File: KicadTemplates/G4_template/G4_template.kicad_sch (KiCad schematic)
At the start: 16 parts, among them J1 Conn_01x04_Female, SW1 SW_SPDT, U1 NUCLEO-G491RE

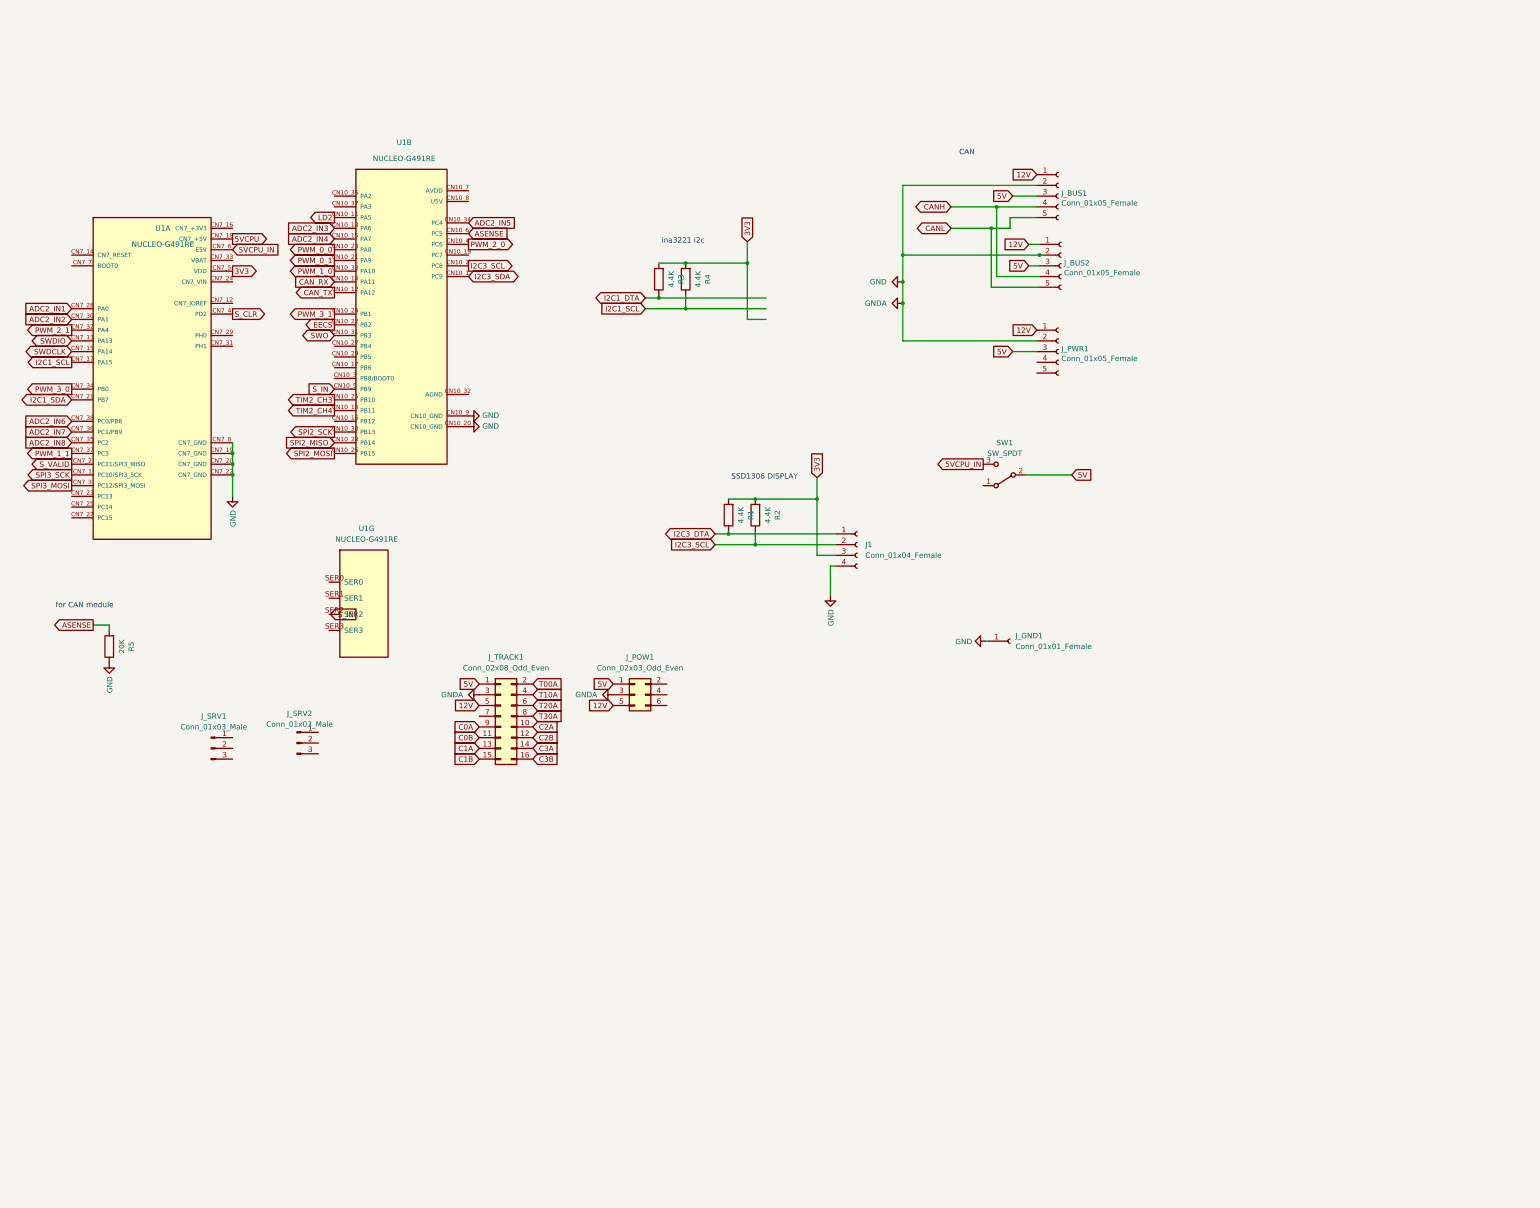
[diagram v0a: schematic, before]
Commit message: update spec POW_CTRL
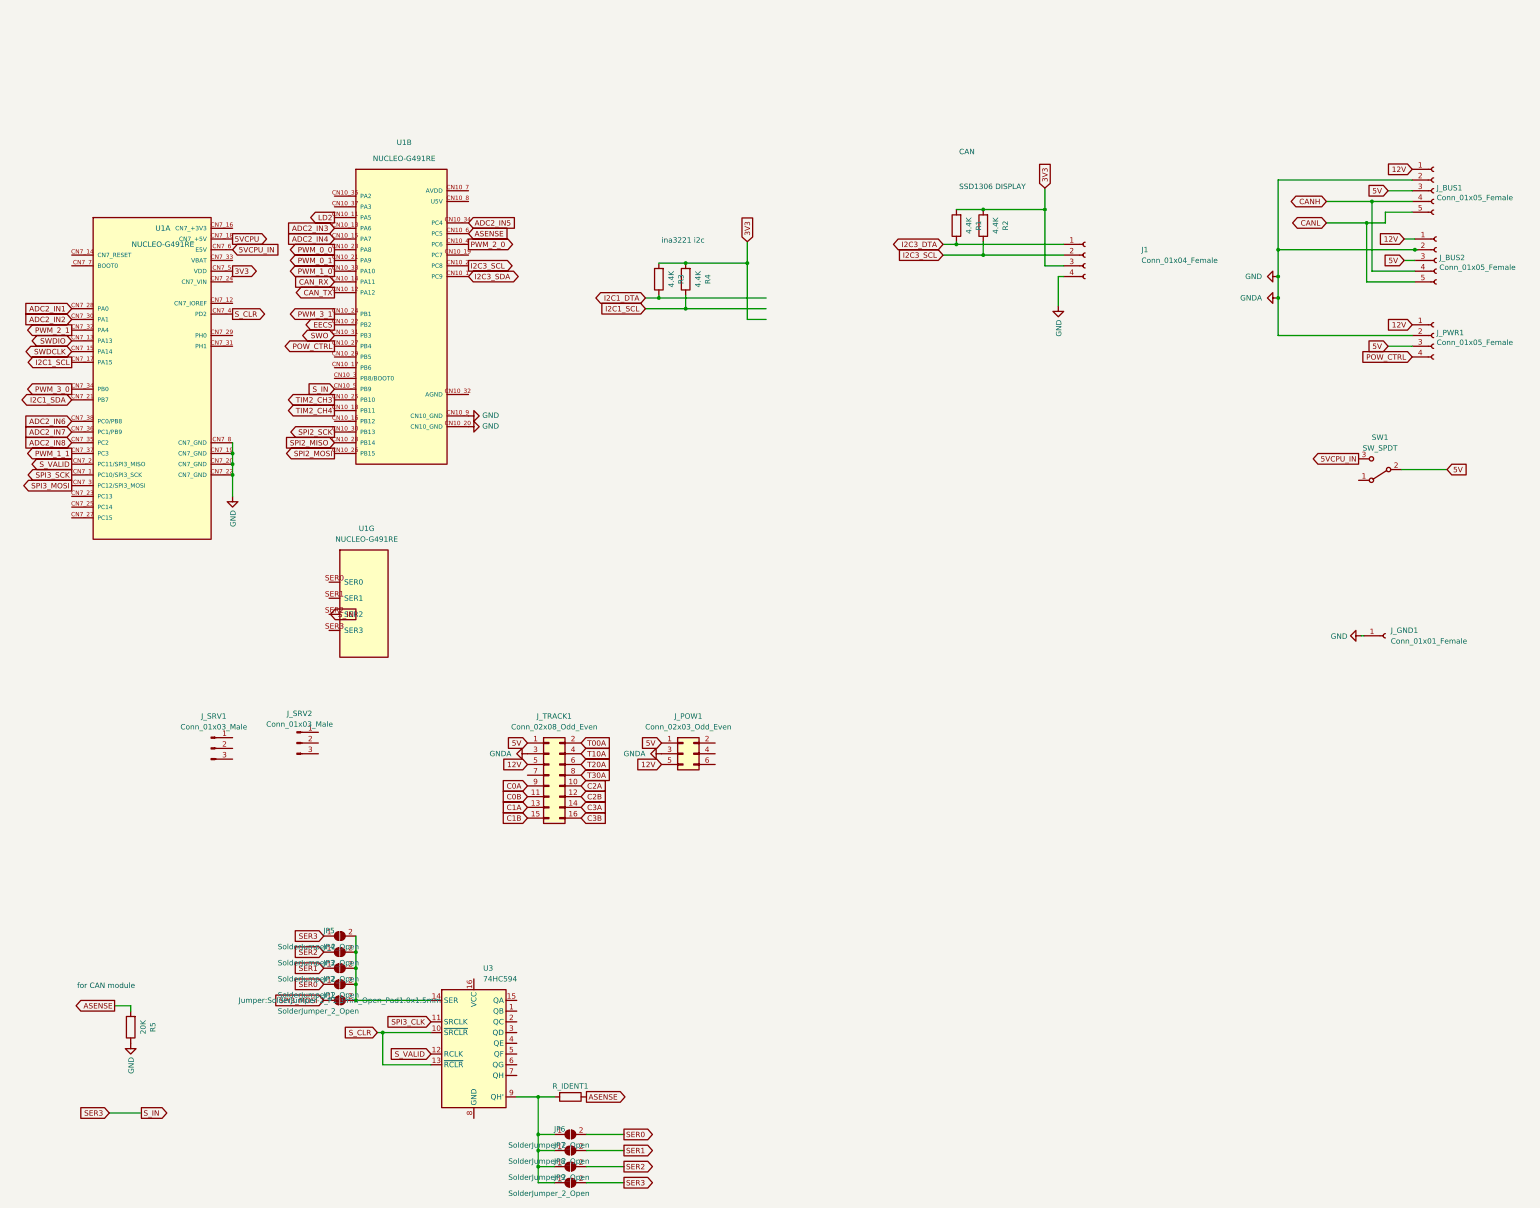
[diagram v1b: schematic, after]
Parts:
- added JP1, JP2, JP3, JP4, JP5, JP6, JP7, JP8, JP9: SolderJumper_2_Open, Jumper:SolderJumper-2_P1.3mm_Open_Pad1.0x1.5mm, symbol Jumper:SolderJumper_2_Open
- added R_IDENT1: ~, Resistor_THT:R_Axial_DIN0207_L6.3mm_D2.5mm_P7.62mm_Horizontal, symbol Device:R
- added U3: 74HC594, Package_DIP:DIP-16_W7.62mm_LongPads, symbol DBN:74HC594
- J_PWR1: footprint Connector_JST:JST_XH_S5B-XH-A_1x05_P2.50mm_Horizontal -> Connector_JST:JST_XH_S4B-XH-A-1_1x04_P2.50mm_Horizontal; symbol Connector:Conn_01x05_Female -> Connector:Conn_01x04_Socket
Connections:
- net ASENSE: now also R_IDENT1.1
- net SPI3_MOSI: now also JP1.1 (A)
- net S_CLR: now also U3.10 (~{SRCLR}), U3.13 (~{RCLR})
- net S_VALID: now also U3.12 (RCLK)
- net POW_CTRL: now reaches J_PWR1.4 (Pin_4)
- net POW_CTRL: now also U1.CN10_27 (PB4)
- net S_IN renamed SER3
- net SER3: now also JP5.1 (A), JP9.2 (B)
- new net: JP6.1 (A), JP7.1 (A), JP8.1 (A), JP9.1 (A), R_IDENT1.2, U3.9 (QH')
- new net: JP1.2 (B), JP2.2 (B), JP3.2 (B), JP4.2 (B), JP5.2 (B), U3.14 (SER)
- new net SER0: JP2.1 (A), JP6.2 (B)
- new net SER1: JP3.1 (A), JP7.2 (B)
- new net SER2: JP4.1 (A), JP8.2 (B)
- new net SPI3_CLK: U3.11 (SRCLK)
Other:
- moved on the sheet: J1, J_BUS1, J_BUS2, J_GND1, J_POW1, J_TRACK1, R1, R2, SW1
